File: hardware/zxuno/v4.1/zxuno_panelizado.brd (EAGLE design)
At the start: 103 parts, among them T1 BC846, U1 6SLX9TQG144, U2 FLASH-SPI-25XXSMD1, U4 AD724, U5 50MHz, U6 3.3V, U7 1.2V, Y1 3.58M, Y2 4.43M

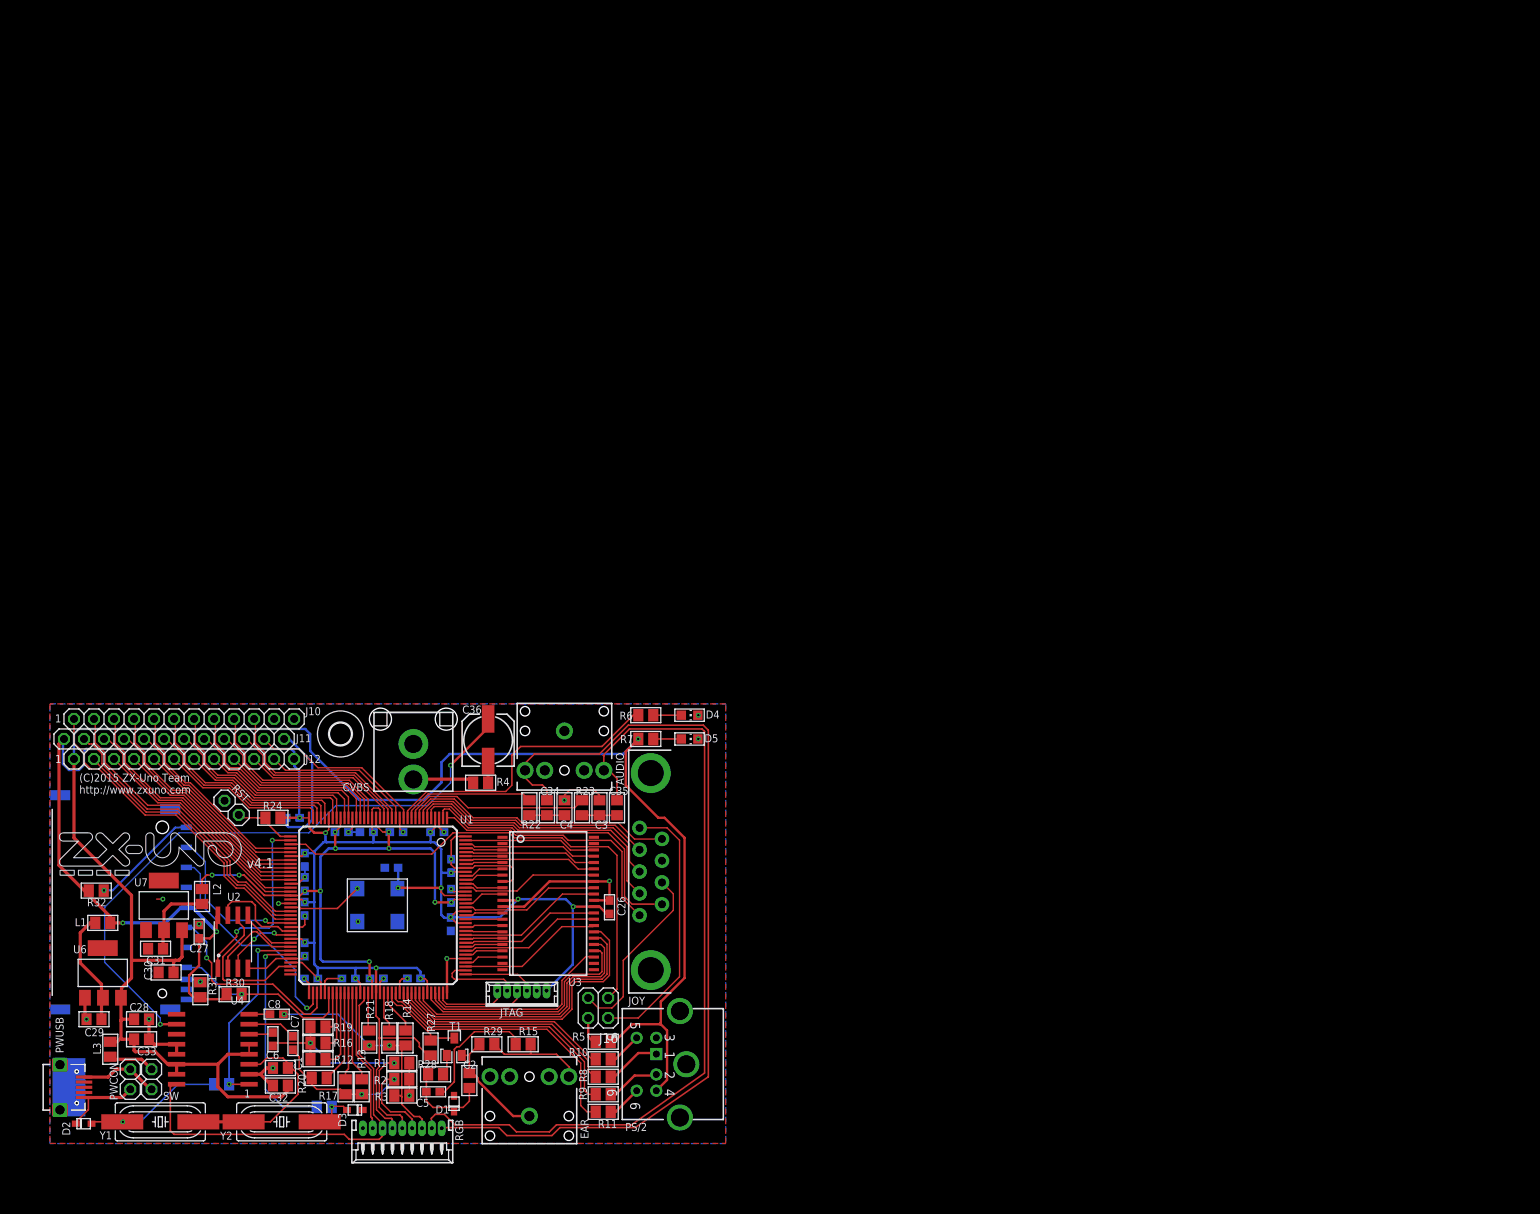
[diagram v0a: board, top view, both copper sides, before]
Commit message: Replico el circuito por 4 wire 0 (0 0) (190 0) (190 150) (0 150) (0 0) wire 0 (0 10) (190 10) wire 0 (0 140) (190 140)
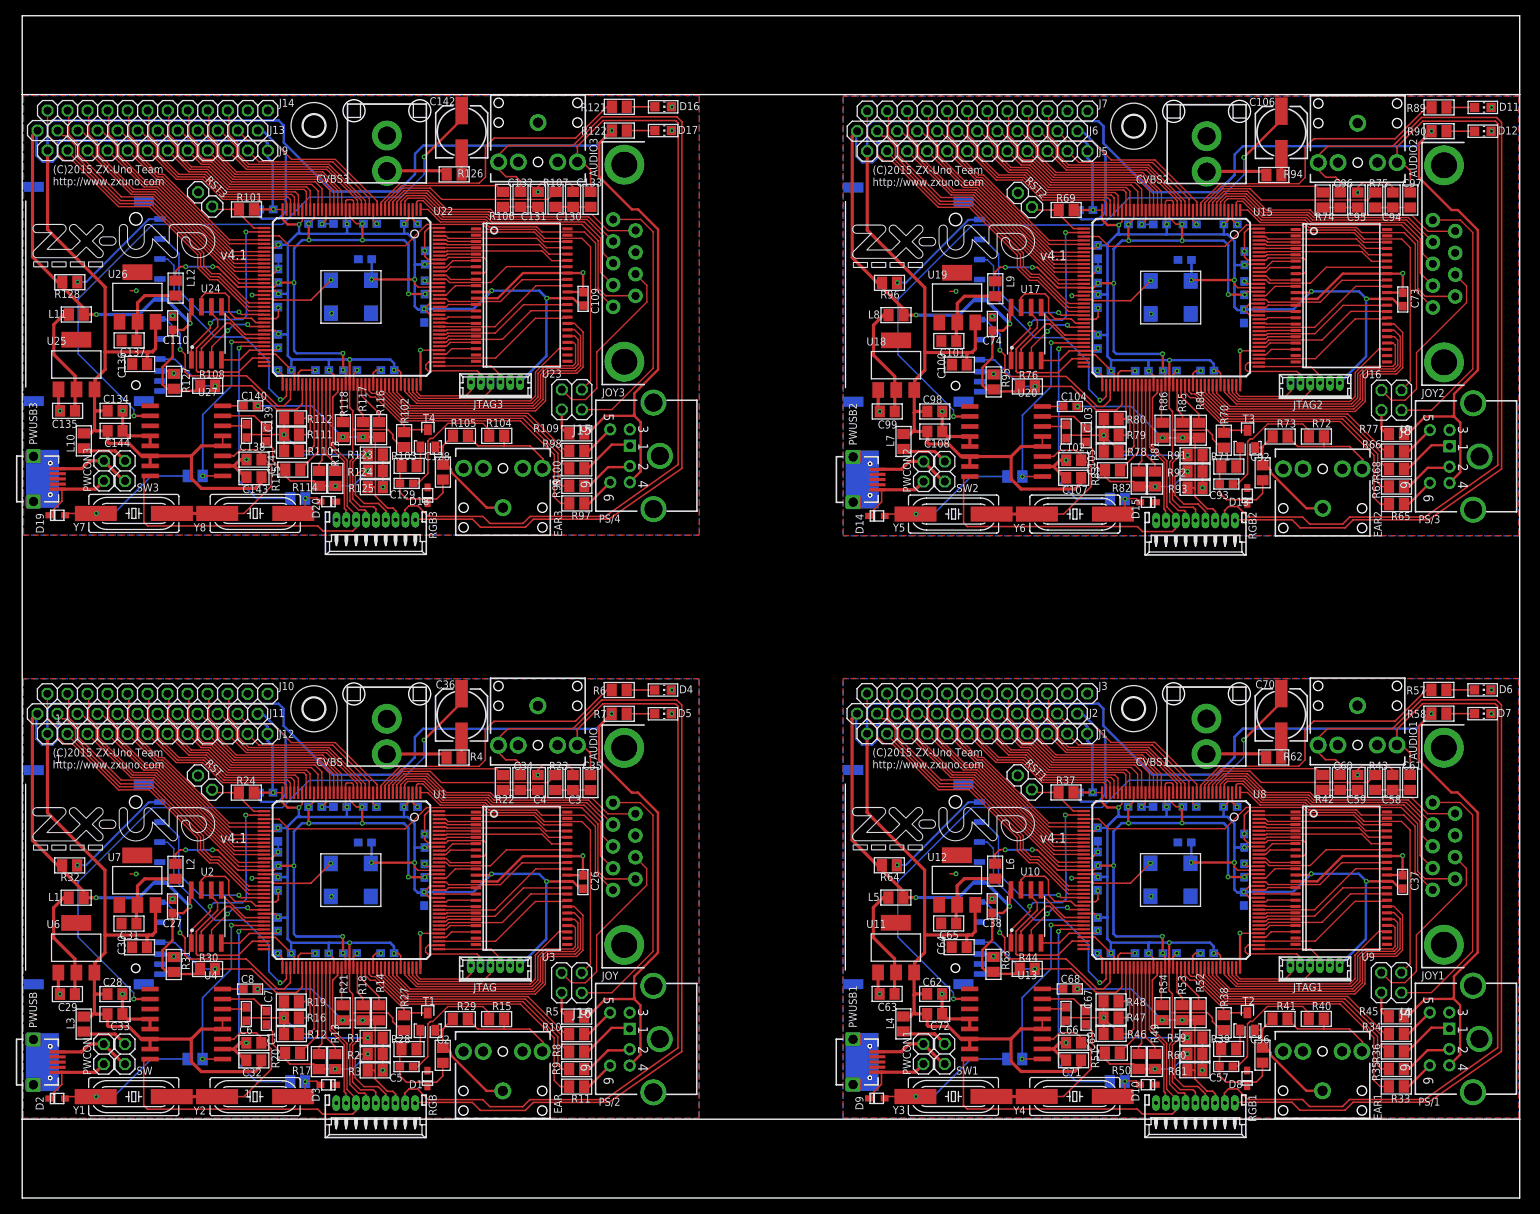
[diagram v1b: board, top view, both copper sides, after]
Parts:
- added AUDIO1, AUDIO2, AUDIO3: Audio, SparkFun-Connectors:AUDIO-JACK
- added C100, C101, C107, C108, C132, C133, C134, C135, C136, C137, C143, C144, C60, C61, C62, C63, C64, C65, C71, C72, C96, C97, C98, C99: 10uF, rcl:C0805
- added C102, C103, C104, C109, C110, C111, C112, C113, C114, C115, C116, C117, C118, C119, C120, C121, C122, C123, C124, C125, C126, C127, C129, C138, C139, C140, C37, C38, C39, C40, C41, C42, C43, C44, C45, C46, C47, C48, C49, C50, C51, C52, C53, C54, C55, C57, C66, C67, C68, C73, C74, C75, C76, C77, C78, C79, C80, C81, C82, C83, C84, C85, C86, C87, C88, C89, C90, C91, C93: 100nF, rcl:C0603
- added C105, C141, C69: 7.5pF, rcl:C0805
- added C106, C142, C70: 220uF, rcl:153CLV-0605
- added C128, C130, C131, C56, C58, C59, C92, C94, C95: 10nF, rcl:C0805
- added CVBS1, CVBS2, CVBS3: RCA, uzebox:RCA
- added D10, D13, D14, D15, D18, D19, D20, D8, D9: (no value), adafruit:SOD-323F
- added D11, D12, D16, D17, D6, D7: (no value), led:CHIP-LED0805
- added EAR1, EAR2, EAR3: EAR, SparkFun-Connectors:AUDIO-JACK
- added H2, H3, H4: MOUNT-HOLE2.8, holes:2,8
- added J1, J13, J14, J2, J3, J5, J6, J7, J9: (no value), pinhead:1X12
- added J15, J4, J8: (no value), pinhead:2X02
- added JOY1, JOY2, JOY3: (no value), SparkFun-Connectors:DB9_MALE
- added JTAG1, JTAG2, JTAG3: JTAG, con-molex:53047-06
- added L10, L11, L12, L4, L5, L6, L7, L8, L9: (no value), rcl:M0805
- added PS/1, PS/3, PS/4: PS/2 Keyb, ZX_UNO_0_14:DINC/MIN_TM/6_1PRIMARY
- added PWCON1, PWCON2, PWCON3, RST1, RST2, RST3, SW1, SW2, SW3: (no value), pinhead:1X02
- added PWUSB1, PWUSB2, PWUSB3: MICROUSB, zxuno_rev_mcleod:MICRO_USB_1PRIMARY
- added R100, R104, R109, R110, R113, R116, R121, R122, R33, R34, R35, R36, R40, R45, R46, R49, R52, R57, R58, R65, R66, R67, R68, R72, R77, R78, R81, R84, R89, R90, R97, R98, R99: 510, rcl:M0805
- added R101, R106, R107, R112, R115, R118, R37, R42, R43, R48, R51, R54, R69, R74, R75, R80, R83, R86: 2K, rcl:M0805
- added R102, R103, R105, R108, R119, R120, R127, R128, R38, R39, R41, R44, R55, R56, R63, R64, R70, R71, R73, R76, R87, R88, R95, R96: 10K, rcl:M0805
- added R111, R114, R117, R47, R50, R53, R79, R82, R85: 1K, rcl:M0805
- added R123, R124, R125, R126, R59, R60, R61, R62, R91, R92, R93, R94: 75, rcl:M0805
- added RGB1, RGB2, RGB3: RGB, con-molex:53048-09
- added SDCARD1, SDCARD2, SDCARD3: (no value), zxuno_rev_mcleod:SDCMF-10915W010
- added T2, T3, T4: BC846, transistor:SOT23
- added U10, U17, U24: FLASH-SPI-25XXSMD1, GadgetFactory:SO08-EIAJ
- added U11, U18, U25: 3.3V, burr-brown:SOT223
- added U12, U19, U26: 1.2V, burr-brown:SOT223
- added U13, U20, U27: AD724, ad725:SO16W
- added U14, U21, U28: 50MHz, ZX_UNO_0_15:SM/OSC_1PRIMARY
- added U15, U22, U8: 6SLX9TQG144, xilinx_devices_V6:TQ144
- added U16, U23, U9: (no value), GadgetFactory:TSOP44-II
- added Y3, Y5, Y7: 3.58M, crystal:HC49UP
- added Y4, Y6, Y8: 4.43M, crystal:HC49UP
- moved C26 4.65 mm to (71.1, 40.1)
- moved D4 4.65 mm to (81.3, 64.5)
- moved D5 4.65 mm to (81.3, 61.4)
- moved JOY 4.65 mm to (76.4, 44.6)
- moved R10 4.65 mm to (70.3, 20.8)
- moved R11 4.65 mm to (70.3, 14.1)
- moved R5 4.65 mm to (70.3, 23.0)
- moved R8 4.65 mm to (70.3, 18.6)
- moved R9 4.65 mm to (70.3, 16.4)
- moved AUDIO 4.65 mm to (65.4, 62.5)
- moved C11 4.65 mm to (51.0, 41.5)
- moved C13 4.65 mm to (32.5, 43.0)
- moved C23 4.65 mm to (32.5, 46.1)
- moved C34 4.65 mm to (63.2, 52.7)
- moved C35 4.65 mm to (72.1, 52.7)
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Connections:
- new net 1.2V1: C39.2, C40.2, C41.2, C42.2, C43.2, L6.2, U8.P128, U8.P19, U8.P28, U8.P52, U8.P89
- new net 1.2V2: C75.2, C76.2, C77.2, C78.2, C79.2, L9.2, U15.P128, U15.P19, U15.P28, U15.P52, U15.P89
- new net 1.2V3: C111.2, C112.2, C113.2, C114.2, C115.2, L12.2, U22.P128, U22.P19, U22.P28, U22.P52, U22.P89
- new net 3.3V1: C37.1, C38.2, C44.2, C45.2, C46.2, C47.2, C48.2, C49.2, C50.2, C51.2, C52.2, C53.2, C54.2, C55.2, J1.12, J2.1, JTAG1.1, L5.2, R37.2, R38.2, R44.1, R63.2, R64.2, RGB1.4, SDCARD1.4, U10.8, U14.4, U8.P103, U8.P122, U8.P125, U8.P129, U8.P135, U8.P18, U8.P20, U8.P31, U8.P36, U8.P4, U8.P42, U8.P53, U8.P63, U8.P69, U8.P76, U8.P86, U8.P90, U9.11, U9.33
- new net 3.3V2: C73.1, C74.2, C80.2, C81.2, C82.2, C83.2, C84.2, C85.2, C86.2, C87.2, C88.2, C89.2, C90.2, C91.2, J5.12, J6.1, JTAG2.1, L8.2, R69.2, R70.2, R76.1, R95.2, R96.2, RGB2.4, SDCARD2.4, U15.P103, U15.P122, U15.P125, U15.P129, U15.P135, U15.P18, U15.P20, U15.P31, U15.P36, U15.P4, U15.P42, U15.P53, U15.P63, U15.P69, U15.P76, U15.P86, U15.P90, U16.11, U16.33, U17.8, U21.4
- new net 3.3V3: C109.1, C110.2, C116.2, C117.2, C118.2, C119.2, C120.2, C121.2, C122.2, C123.2, C124.2, C125.2, C126.2, C127.2, J13.1, J9.12, JTAG3.1, L11.2, R101.2, R102.2, R108.1, R127.2, R128.2, RGB3.4, SDCARD3.4, U22.P103, U22.P122, U22.P125, U22.P129, U22.P135, U22.P18, U22.P20, U22.P31, U22.P36, U22.P4, U22.P42, U22.P53, U22.P63, U22.P69, U22.P76, U22.P86, U22.P90, U23.11, U23.33, U24.8, U28.4
- new net 5V1: C62.1, C64.1, C71.2, C72.2, J1.1, L4.2, PS/1.4, R45.1, R58.2, U11.3, U12.3, U13.14, U13.15, U13.4, U13.5
- new net 5V2: C100.1, C107.2, C108.2, C98.1, J5.1, L7.2, PS/3.4, R77.1, R90.2, U18.3, U19.3, U20.14, U20.15, U20.4, U20.5
- new net 5V3: C134.1, C136.1, C143.2, C144.2, J9.1, L10.2, PS/4.4, R109.1, R122.2, U25.3, U26.3, U27.14, U27.15, U27.4, U27.5
- new net AUDIO_LEFT1: R42.2, U8.P10
- new net AUDIO_LEFT2: R74.2, U15.P10
- new net AUDIO_LEFT3: R106.2, U22.P10
- new net AUDIO_RIGHT1: R43.2, U8.P9
- new net AUDIO_RIGHT2: R75.2, U15.P9
- new net AUDIO_RIGHT3: R107.2, U22.P9
- new net B10: C104.2, R84.1, R85.1, R86.1, R93.1, RGB2.7
- new net B11: R118.2, U22.P88
- new net B12: R117.2, U22.P92
- new net B13: R116.2, U22.P93
- new net B14: C140.2, R116.1, R117.1, R118.1, R125.1, RGB3.7
- new net B3: R54.2, U8.P88
- new net B4: R53.2, U8.P92
- new net B5: R52.2, U8.P93
- new net B6: C68.2, R52.1, R53.1, R54.1, R61.1, RGB1.7
- new net B7: R86.2, U15.P88
- new net B8: R85.2, U15.P92
- new net B9: R84.2, U15.P93
- new net CLK1: U14.3, U8.P55
- new net CLK2: U15.P55, U21.3
- new net CLK3: U22.P55, U28.3
- new net CSYNC1: RGB1.3, U13.16, U8.P87
- new net CSYNC2: RGB2.3, U15.P87, U20.16
- new net CSYNC3: RGB3.3, U22.P87, U27.16
- new net EAR1: R38.1, T2.3, U8.P94
- new net EAR2: R70.1, T3.3, U15.P94
- new net EAR3: R102.1, T4.3, U22.P94
- new net EXT1: J1.2, U8.P57
- new net EXT100: J9.5, U22.P43
- new net EXT101: J13.5, U22.P41
- new net EXT102: J14.5, U22.P40
- new net EXT103: J9.6, U22.P35
- new net EXT104: J13.6, U22.P34
- new net EXT105: J14.6, U22.P33
- new net EXT106: J9.7, U22.P32
- new net EXT107: J13.7, U22.P30
- new net EXT108: J14.7, U22.P29
- new net EXT109: J9.8, U22.P27
- new net EXT110: J13.8, U22.P26
- new net EXT111: J14.8, U22.P24
- new net EXT112: J9.9, U22.P23
- new net EXT113: J13.9, U22.P22
- new net EXT114: J14.9, U22.P21
- new net EXT115: J9.10, U22.P17
- new net EXT116: J13.10, U22.P16
- new net EXT117: J14.10, U22.P15
- new net EXT118: J9.11, U22.P14
- new net EXT119: J13.11, U22.P12
- new net EXT120: J14.1, U22.P58
- new net EXT2: J2.2, U8.P56
- new net EXT3: J3.2, U8.P51
- new net EXT36: J3.3, U8.P47
- new net EXT37: J1.4, U8.P46
- new net EXT38: J2.4, U8.P45
- new net EXT39: J3.4, U8.P44
- new net EXT4: J1.3, U8.P50
- new net EXT40: J1.5, U8.P43
- new net EXT41: J2.5, U8.P41
- new net EXT42: J3.5, U8.P40
- new net EXT43: J1.6, U8.P35
- new net EXT44: J2.6, U8.P34
- new net EXT45: J3.6, U8.P33
- new net EXT46: J1.7, U8.P32
- new net EXT47: J2.7, U8.P30
- new net EXT48: J3.7, U8.P29
- new net EXT49: J1.8, U8.P27
- new net EXT5: J2.3, U8.P48
- new net EXT50: J2.8, U8.P26
- new net EXT51: J3.8, U8.P24
- new net EXT52: J1.9, U8.P23
- new net EXT53: J2.9, U8.P22
- new net EXT54: J3.9, U8.P21
- new net EXT55: J1.10, U8.P17
- new net EXT56: J2.10, U8.P16
- new net EXT57: J3.10, U8.P15
- new net EXT58: J1.11, U8.P14
- new net EXT59: J2.11, U8.P12
- new net EXT60: J3.1, U8.P58
- new net EXT61: J5.2, U15.P57
- new net EXT62: J6.2, U15.P56
- new net EXT63: J7.2, U15.P51
- new net EXT64: J5.3, U15.P50
- new net EXT65: J6.3, U15.P48
- new net EXT66: J7.3, U15.P47
- new net EXT67: J5.4, U15.P46
- new net EXT68: J6.4, U15.P45
- new net EXT69: J7.4, U15.P44
- new net EXT70: J5.5, U15.P43
- new net EXT71: J6.5, U15.P41
- new net EXT72: J7.5, U15.P40
- new net EXT73: J5.6, U15.P35
- new net EXT74: J6.6, U15.P34
- new net EXT75: J7.6, U15.P33
- new net EXT76: J5.7, U15.P32
- new net EXT77: J6.7, U15.P30
- new net EXT78: J7.7, U15.P29
- new net EXT79: J5.8, U15.P27
- new net EXT80: J6.8, U15.P26
- new net EXT81: J7.8, U15.P24
- new net EXT82: J5.9, U15.P23
- new net EXT83: J6.9, U15.P22
- new net EXT84: J7.9, U15.P21
- new net EXT85: J5.10, U15.P17
- new net EXT86: J6.10, U15.P16
- new net EXT87: J7.10, U15.P15
- new net EXT88: J5.11, U15.P14
- new net EXT89: J6.11, U15.P12
- new net EXT90: J7.1, U15.P58
- new net EXT91: J9.2, U22.P57
- new net EXT92: J13.2, U22.P56
- new net EXT93: J14.2, U22.P51
- new net EXT94: J9.3, U22.P50
- new net EXT95: J13.3, U22.P48
- new net EXT96: J14.3, U22.P47
- new net EXT97: J9.4, U22.P46
- new net EXT98: J13.4, U22.P45
- new net EXT99: J14.4, U22.P44
- new net FLASH_CS1: U10.1, U8.P38
- new net FLASH_CS2: U15.P38, U17.1
- new net FLASH_CS3: U22.P38, U24.1
- new net FLASH_HOLD1: U10.7, U8.P61
- new net FLASH_HOLD2: U15.P61, U17.7
- new net FLASH_HOLD3: U22.P61, U24.7
- new net FLASH_MISO1: U10.2, U8.P65
- new net FLASH_MISO2: U15.P65, U17.2
- new net FLASH_MISO3: U22.P65, U24.2
- new net FLASH_MOSI1: U10.5, U8.P64
- new net FLASH_MOSI2: U15.P64, U17.5
- new net FLASH_MOSI3: U22.P64, U24.5
- new net FLASH_SCK1: U10.6, U8.P70
- new net FLASH_SCK2: U15.P70, U17.6
- new net FLASH_SCK3: U22.P70, U24.6
- new net FLASH_WP1: U10.3, U8.P62
- new net FLASH_WP2: U15.P62, U17.3
- new net FLASH_WP3: U22.P62, U24.3
- new net G10: C103.2, R81.1, R82.1, R83.1, R92.1, RGB2.6
- new net G11: R115.2, U22.P82
- new net G12: R114.2, U22.P83
- new net G13: R113.2, U22.P84
- new net G14: C139.2, R113.1, R114.1, R115.1, R124.1, RGB3.6
- new net G3: R51.2, U8.P82
- new net G4: R50.2, U8.P83
- new net G5: R49.2, U8.P84
- new net G6: C67.2, R49.1, R50.1, R51.1, R60.1, RGB1.6
- new net G7: R83.2, U15.P82
- new net G8: R82.2, U15.P83
- new net G9: R81.2, U15.P84
- new net GND1: AUDIO1.SLEEVE, C37.2, C38.1, C39.1, C40.1, C41.1, C42.1, C43.1, C44.1, C45.1, C46.1, C47.1, C48.1, C49.1, C50.1, C51.1, C52.1, C53.1, C54.1, C55.1, C56.2, C58.2, C59.2, C62.2, C63.2, C64.2, C65.2, C69.2, C71.1, C72.1, CVBS1.GND, D10.C, D6.C, D7.C, D8.A, D9.C, EAR1.SLEEVE, J2.12, J3.12, JOY1.8, JTAG1.2, PS/1.3, PWCON1.1, PWUSB1.5, R41.2, R59.2, R60.2, R61.2, RGB1.1, RST1.1, SDCARD1.3, SDCARD1.6, SDCARD1.M1, SDCARD1.M2, SDCARD1.M3, SDCARD1.M4, T2.2, U10.4, U11.1, U12.1, U13.12, U13.13, U13.2, U14.2, U8.P108, U8.P113, U8.P13, U8.P130, U8.P136, U8.P144, U8.P25, U8.P3, U8.P49, U8.P54, U8.P60, U8.P68, U8.P73, U8.P77, U8.P91, U8.P96, U9.12, U9.34, U9.37, U9.8
- new net GND2: AUDIO2.SLEEVE, C100.2, C101.2, C105.2, C107.1, C108.1, C73.2, C74.1, C75.1, C76.1, C77.1, C78.1, C79.1, C80.1, C81.1, C82.1, C83.1, C84.1, C85.1, C86.1, C87.1, C88.1, C89.1, C90.1, C91.1, C92.2, C94.2, C95.2, C98.2, C99.2, CVBS2.GND, D11.C, D12.C, D13.A, D14.C, D15.C, EAR2.SLEEVE, J6.12, J7.12, JOY2.8, JTAG2.2, PS/3.3, PWCON2.1, PWUSB2.5, R73.2, R91.2, R92.2, R93.2, RGB2.1, RST2.1, SDCARD2.3, SDCARD2.6, SDCARD2.M1, SDCARD2.M2, SDCARD2.M3, SDCARD2.M4, T3.2, U15.P108, U15.P113, U15.P13, U15.P130, U15.P136, U15.P144, U15.P25, U15.P3, U15.P49, U15.P54, U15.P60, U15.P68, U15.P73, U15.P77, U15.P91, U15.P96, U16.12, U16.34, U16.37, U16.8, U17.4, U18.1, U19.1, U20.12, U20.13, U20.2, U21.2
- new net GND3: AUDIO3.SLEEVE, C109.2, C110.1, C111.1, C112.1, C113.1, C114.1, C115.1, C116.1, C117.1, C118.1, C119.1, C120.1, C121.1, C122.1, C123.1, C124.1, C125.1, C126.1, C127.1, C128.2, C130.2, C131.2, C134.2, C135.2, C136.2, C137.2, C141.2, C143.1, C144.1, CVBS3.GND, D16.C, D17.C, D18.A, D19.C, D20.C, EAR3.SLEEVE, J13.12, J14.12, JOY3.8, JTAG3.2, PS/4.3, PWCON3.1, PWUSB3.5, R105.2, R123.2, R124.2, R125.2, RGB3.1, RST3.1, SDCARD3.3, SDCARD3.6, SDCARD3.M1, SDCARD3.M2, SDCARD3.M3, SDCARD3.M4, T4.2, U22.P108, U22.P113, U22.P13, U22.P130, U22.P136, U22.P144, U22.P25, U22.P3, U22.P49, U22.P54, U22.P60, U22.P68, U22.P73, U22.P77, U22.P91, U22.P96, U23.12, U23.34, U23.37, U23.8, U24.4, U25.1, U26.1, U27.12, U27.13, U27.2, U28.2
- new net JOY_DOWN1: JOY1.2, U8.P5
- new net JOY_DOWN2: JOY2.2, U15.P5
- new net JOY_DOWN3: JOY3.2, U22.P5
- new net JOY_FIRE10: JOY3.6, U22.P2
- new net JOY_FIRE11: JOY3.9, U22.P8
- new net JOY_FIRE12: J15.1, U22.P39
- new net JOY_FIRE4: JOY1.6, U8.P2
- new net JOY_FIRE5: JOY1.9, U8.P8
- new net JOY_FIRE6: J4.1, U8.P39
- new net JOY_FIRE7: JOY2.6, U15.P2
- new net JOY_FIRE8: JOY2.9, U15.P8
- new net JOY_FIRE9: J8.1, U15.P39
- new net JOY_LEFT1: JOY1.3, U8.P6
- new net JOY_LEFT2: JOY2.3, U15.P6
- new net JOY_LEFT3: JOY3.3, U22.P6
- new net JOY_RIGHT1: JOY1.4, U8.P7
- new net JOY_RIGHT2: JOY2.4, U15.P7
- new net JOY_RIGHT3: JOY3.4, U22.P7
- new net JOY_UP1: JOY1.1, U8.P1
- new net JOY_UP2: JOY2.1, U15.P1
- new net JOY_UP3: JOY3.1, U22.P1
- new net L-OUT1: AUDIO1.TIP, C60.2, RGB1.9
- new net L-OUT2: AUDIO2.TIP, C96.2, RGB2.9
- new net L-OUT3: AUDIO3.TIP, C132.2, RGB3.9
- new net LED1: R57.2, U8.P11
- new net LED2: R89.2, U15.P11
- new net LED3: R121.2, U22.P11
- new net N$100: C135.1, L11.1, U25.2
- new net N$101: C137.1, L12.1, U26.2
- new net N$102: C139.1, U27.7
- new net N$103: C138.1, U27.6
- new net N$104: C141.1, U27.3, Y7.2, Y8.2
- new net N$105: D20.A, R120.1, Y8.1
- new net N$106: D19.A, R119.2, Y7.1
- new net N$107: C142.+, U27.10
- new net N$108: C140.1, U27.8
- new net N$109: C142.-, R126.1
- new net N$110: CVBS3.SIG, R126.2
- new net N$111: D16.A, R121.1
- new net N$112: D17.A, R122.1
- new net N$113: R101.1, RST3.2, U22.P37
- new net N$114: R127.1, SDCARD3.8
- new net N$115: R128.1, SDCARD3.9
- new net N$116: J15.4, R109.2
- new net N$16: PS/1.6, R33.1
- new net N$29: PS/1.5, R34.1
- new net N$30: PS/1.2, R35.1
- new net N$33: PS/1.1, R36.1
- new net N$34: R39.2, T2.1
- new net N$35: C56.1, C57.1, D8.C, R39.1
- new net N$36: C57.2, R40.2
- new net N$37: EAR1.TIP, R40.1, R41.1
- new net N$38: C58.1, C61.1, R43.1
- new net N$39: C59.1, C60.1, R42.1
- new net N$40: PWCON1.2, PWUSB1.1, SW1.2
- new net N$41: L4.1, SW1.1
- new net N$42: C63.1, L5.1, U11.2
- new net N$43: C65.1, L6.1, U12.2
- new net N$44: C67.1, U13.7
- new net N$45: C66.1, U13.6
- new net N$46: C69.1, U13.3, Y3.2, Y4.2
- new net N$47: D10.A, R56.1, Y4.1
- new net N$48: D9.A, R55.2, Y3.1
- new net N$49: C70.+, U13.10
- new net N$50: C68.1, U13.8
- new net N$51: C70.-, R62.1
- new net N$52: CVBS1.SIG, R62.2
- new net N$53: D6.A, R57.1
- new net N$54: D7.A, R58.1
- new net N$55: R37.1, RST1.2, U8.P37
- new net N$56: R63.1, SDCARD1.8
- new net N$57: R64.1, SDCARD1.9
- new net N$58: J4.4, R45.2
- new net N$59: PS/3.6, R65.1
- new net N$60: PS/3.5, R66.1
- new net N$61: PS/3.2, R67.1
- new net N$62: PS/3.1, R68.1
- new net N$63: R71.2, T3.1
- new net N$64: C92.1, C93.1, D13.C, R71.1
- new net N$65: C93.2, R72.2
- new net N$66: EAR2.TIP, R72.1, R73.1
- new net N$67: C94.1, C97.1, R75.1
- new net N$68: C95.1, C96.1, R74.1
- new net N$69: PWCON2.2, PWUSB2.1, SW2.2
- new net N$70: L7.1, SW2.1
- new net N$71: C99.1, L8.1, U18.2
- new net N$72: C101.1, L9.1, U19.2
- new net N$73: C103.1, U20.7
- new net N$74: C102.1, U20.6
- new net N$75: C105.1, U20.3, Y5.2, Y6.2
- new net N$76: D15.A, R88.1, Y6.1
- new net N$77: D14.A, R87.2, Y5.1
- new net N$78: C106.+, U20.10
- new net N$79: C104.1, U20.8
- new net N$80: C106.-, R94.1
- new net N$81: CVBS2.SIG, R94.2
- new net N$82: D11.A, R89.1
- new net N$83: D12.A, R90.1
- new net N$84: R69.1, RST2.2, U15.P37
- new net N$85: R95.1, SDCARD2.8
- new net N$86: R96.1, SDCARD2.9
- new net N$87: J8.4, R77.2
- new net N$88: PS/4.6, R97.1
- new net N$89: PS/4.5, R98.1
- new net N$90: PS/4.2, R99.1
- new net N$91: PS/4.1, R100.1
- new net N$92: R103.2, T4.1
- new net N$93: C128.1, C129.1, D18.C, R103.1
- new net N$94: C129.2, R104.2
- new net N$95: EAR3.TIP, R104.1, R105.1
- new net N$96: C130.1, C133.1, R107.1
- new net N$97: C131.1, C132.1, R106.1
- new net N$98: PWCON3.2, PWUSB3.1, SW3.2
- new net N$99: L10.1, SW3.1
- new net PIN1: J4.3, JOY1.7
- new net PIN2: J4.2, JOY1.5
- new net PIN3: J8.3, JOY2.7
- new net PIN4: J8.2, JOY2.5
- new net PIN6: J15.3, JOY3.7
- new net PIN8: J15.2, JOY3.5
- new net PS2_CLK1: R34.2, U8.P99
- new net PS2_CLK2: R66.2, U15.P99
- new net PS2_CLK3: R98.2, U22.P99
- new net PS2_DATA1: R36.2, U8.P98
- new net PS2_DATA2: R68.2, U15.P98
- new net PS2_DATA3: R100.2, U22.P98
- new net PS2_PIN1: R33.2, U8.P95
- new net PS2_PIN3: R35.2, U8.P97
- new net PS2_PIN4: R65.2, U15.P95
- new net PS2_PIN5: R67.2, U15.P97
- new net PS2_PIN7: R97.2, U22.P95
- new net PS2_PIN8: R99.2, U22.P97
- new net R-OUT1: AUDIO1.RING, C61.2, RGB1.8
- new net R-OUT2: AUDIO2.RING, C97.2, RGB2.8
- new net R-OUT3: AUDIO3.RING, C133.2, RGB3.8
- new net R10: C102.2, R78.1, R79.1, R80.1, R91.1, RGB2.5
- new net R11: R112.2, U22.P79
- new net R12: R111.2, U22.P80
- new net R13: R110.2, U22.P81
- new net R14: C138.2, R110.1, R111.1, R112.1, R123.1, RGB3.5
- new net R3: R48.2, U8.P79
- new net R4: R47.2, U8.P80
- new net R5: R46.2, U8.P81
- new net R6: C66.2, R46.1, R47.1, R48.1, R59.1, RGB1.5
- new net R7: R80.2, U15.P79
- new net R8: R79.2, U15.P80
- new net R9: R78.2, U15.P81
- new net SD_CS1: SDCARD1.1, U8.P59
- new net SD_CS2: SDCARD2.1, U15.P59
- new net SD_CS3: SDCARD3.1, U22.P59
- new net SD_MISO1: R44.2, SDCARD1.7, U8.P78
- new net SD_MISO2: R76.2, SDCARD2.7, U15.P78
- new net SD_MISO3: R108.2, SDCARD3.7, U22.P78
- new net SD_MOSI1: SDCARD1.2, U8.P74
- new net SD_MOSI2: SDCARD2.2, U15.P74
- new net SD_MOSI3: SDCARD3.2, U22.P74
- new net SD_SCK1: SDCARD1.5, U8.P75
- new net SD_SCK2: SDCARD2.5, U15.P75
- new net SD_SCK3: SDCARD3.5, U22.P75
- new net STDN1: R55.1, U13.1, U8.P66
- new net STDN2: R87.1, U15.P66, U20.1
- new net STDN3: R119.1, U22.P66, U27.1
- new net STDNB1: R56.2, U8.P67
- new net STDNB2: R88.2, U15.P67
- new net STDNB3: R120.2, U22.P67
- new net TCK1: JTAG1.3, U8.P109
- new net TCK2: JTAG2.3, U15.P109
- new net TCK3: JTAG3.3, U22.P109
- new net TDI1: JTAG1.5, U8.P110
- new net TDI2: JTAG2.5, U15.P110
- new net TDI3: JTAG3.5, U22.P110
- new net TDO1: JTAG1.4, U8.P106
- new net TDO2: JTAG2.4, U15.P106
- new net TDO3: JTAG3.4, U22.P106
- new net TMS1: JTAG1.6, U8.P107
- new net TMS2: JTAG2.6, U15.P107
- new net TMS3: JTAG3.6, U22.P107
- new net VSYNC1: RGB1.2, U8.P85
- new net VSYNC2: RGB2.2, U15.P85
- new net VSYNC3: RGB3.2, U22.P85
- new net WR1: U8.P121, U9.15
- new net WR2: U15.P121, U16.15
- new net WR3: U22.P121, U23.15
- new net XA21: U8.P141, U9.3
- new net XA22: U8.P137, U9.5
- new net XA23: U8.P134, U9.6
- new net XA24: U8.P133, U9.7
- new net XA25: U8.P120, U9.16
- new net XA26: U8.P118, U9.17
- new net XA27: U8.P116, U9.18
- new net XA28: U8.P114, U9.19
- new net XA29: U8.P112, U9.20
- new net XA30: U8.P104, U9.26
- new net XA31: U8.P102, U9.27
- new net XA32: U8.P101, U9.28
- new net XA33: U8.P100, U9.29
- new net XA34: U8.P111, U9.30
- new net XA35: U8.P131, U9.38
- new net XA36: U8.P138, U9.39
- new net XA37: U8.P140, U9.40
- new net XA38: U8.P142, U9.41
- new net XA39: U8.P105, U9.25
- new net XA40: U8.P143, U9.42
- new net XA41: U8.P139, U9.4
- new net XA42: U15.P141, U16.3
- new net XA43: U15.P137, U16.5
- new net XA44: U15.P134, U16.6
- new net XA45: U15.P133, U16.7
- new net XA46: U15.P120, U16.16
- new net XA47: U15.P118, U16.17
- new net XA48: U15.P116, U16.18
- new net XA49: U15.P114, U16.19
- new net XA50: U15.P112, U16.20
- new net XA51: U15.P104, U16.26
- new net XA52: U15.P102, U16.27
- new net XA53: U15.P101, U16.28
- new net XA54: U15.P100, U16.29
- new net XA55: U15.P111, U16.30
- new net XA56: U15.P131, U16.38
- new net XA57: U15.P138, U16.39
- new net XA58: U15.P140, U16.40
- new net XA59: U15.P142, U16.41
- new net XA60: U15.P105, U16.25
- new net XA61: U15.P143, U16.42
- new net XA62: U15.P139, U16.4
- new net XA63: U22.P141, U23.3
- new net XA64: U22.P137, U23.5
- new net XA65: U22.P134, U23.6
- new net XA66: U22.P133, U23.7
- new net XA67: U22.P120, U23.16
- new net XA68: U22.P118, U23.17
- new net XA69: U22.P116, U23.18
- new net XA70: U22.P114, U23.19
- new net XA71: U22.P112, U23.20
- new net XA72: U22.P104, U23.26
- new net XA73: U22.P102, U23.27
- new net XA74: U22.P101, U23.28
- new net XA75: U22.P100, U23.29
- new net XA76: U22.P111, U23.30
- new net XA77: U22.P131, U23.38
- new net XA78: U22.P138, U23.39
- new net XA79: U22.P140, U23.40
- new net XA80: U22.P142, U23.41
- new net XA81: U22.P105, U23.25
- new net XA82: U22.P143, U23.42
- new net XA83: U22.P139, U23.4
- new net XD10: U8.P124, U9.13
- new net XD11: U8.P123, U9.14
- new net XD12: U8.P115, U9.31
- new net XD13: U8.P117, U9.32
- new net XD14: U8.P119, U9.35
- new net XD15: U8.P126, U9.36
- new net XD16: U15.P132, U16.9
- new net XD17: U15.P127, U16.10
- new net XD18: U15.P124, U16.13
- new net XD19: U15.P123, U16.14
- new net XD20: U15.P115, U16.31
- new net XD21: U15.P117, U16.32
- new net XD22: U15.P119, U16.35
- new net XD23: U15.P126, U16.36
- new net XD24: U22.P132, U23.9
- new net XD25: U22.P127, U23.10
- new net XD26: U22.P124, U23.13
- new net XD27: U22.P123, U23.14
- new net XD28: U22.P115, U23.31
- new net XD29: U22.P117, U23.32
- new net XD30: U22.P119, U23.35
- new net XD31: U22.P126, U23.36
- new net XD8: U8.P132, U9.9
- new net XD9: U8.P127, U9.10
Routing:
- net 3.3V2: track 0.00 -> 288.5 mm, vias 0 -> 19
- net 3.3V3: track 0.00 -> 288.5 mm, vias 0 -> 19
- net 3.3V1: track 0.00 -> 288.5 mm, vias 0 -> 19
- net 5V3: track 0.00 -> 233.3 mm, vias 0 -> 1
- net 5V1: track 0.00 -> 233.3 mm, vias 0 -> 1
- net 5V2: track 0.00 -> 233.3 mm, vias 0 -> 1
- net GND3: track 0.00 -> 149.1 mm, vias 0 -> 25
- net GND2: track 0.00 -> 149.1 mm, vias 0 -> 25
- net GND1: track 0.00 -> 149.1 mm, vias 0 -> 25
- net L-OUT2: track 0.00 -> 112.9 mm
- net L-OUT1: track 0.00 -> 112.9 mm
- net L-OUT3: track 0.00 -> 112.9 mm
- net R-OUT2: track 0.00 -> 104.1 mm
- net R-OUT3: track 0.00 -> 104.1 mm
- net R-OUT1: track 0.00 -> 104.1 mm
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- added copper zone on layer 1, net GND1
- added copper zone on layer 16, net GND1
- added copper zone on layer 1, net GND2
- added copper zone on layer 16, net GND2
- added copper zone on layer 1, net GND3
- added copper zone on layer 16, net GND3
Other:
- board outline added: 190 x 150 mm

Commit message: wire 0 (0 66) (190 66) wire 0 (0 84) (190 84) wire 0 (86 10) (86 140) wire 0 (104 10) (104 140)
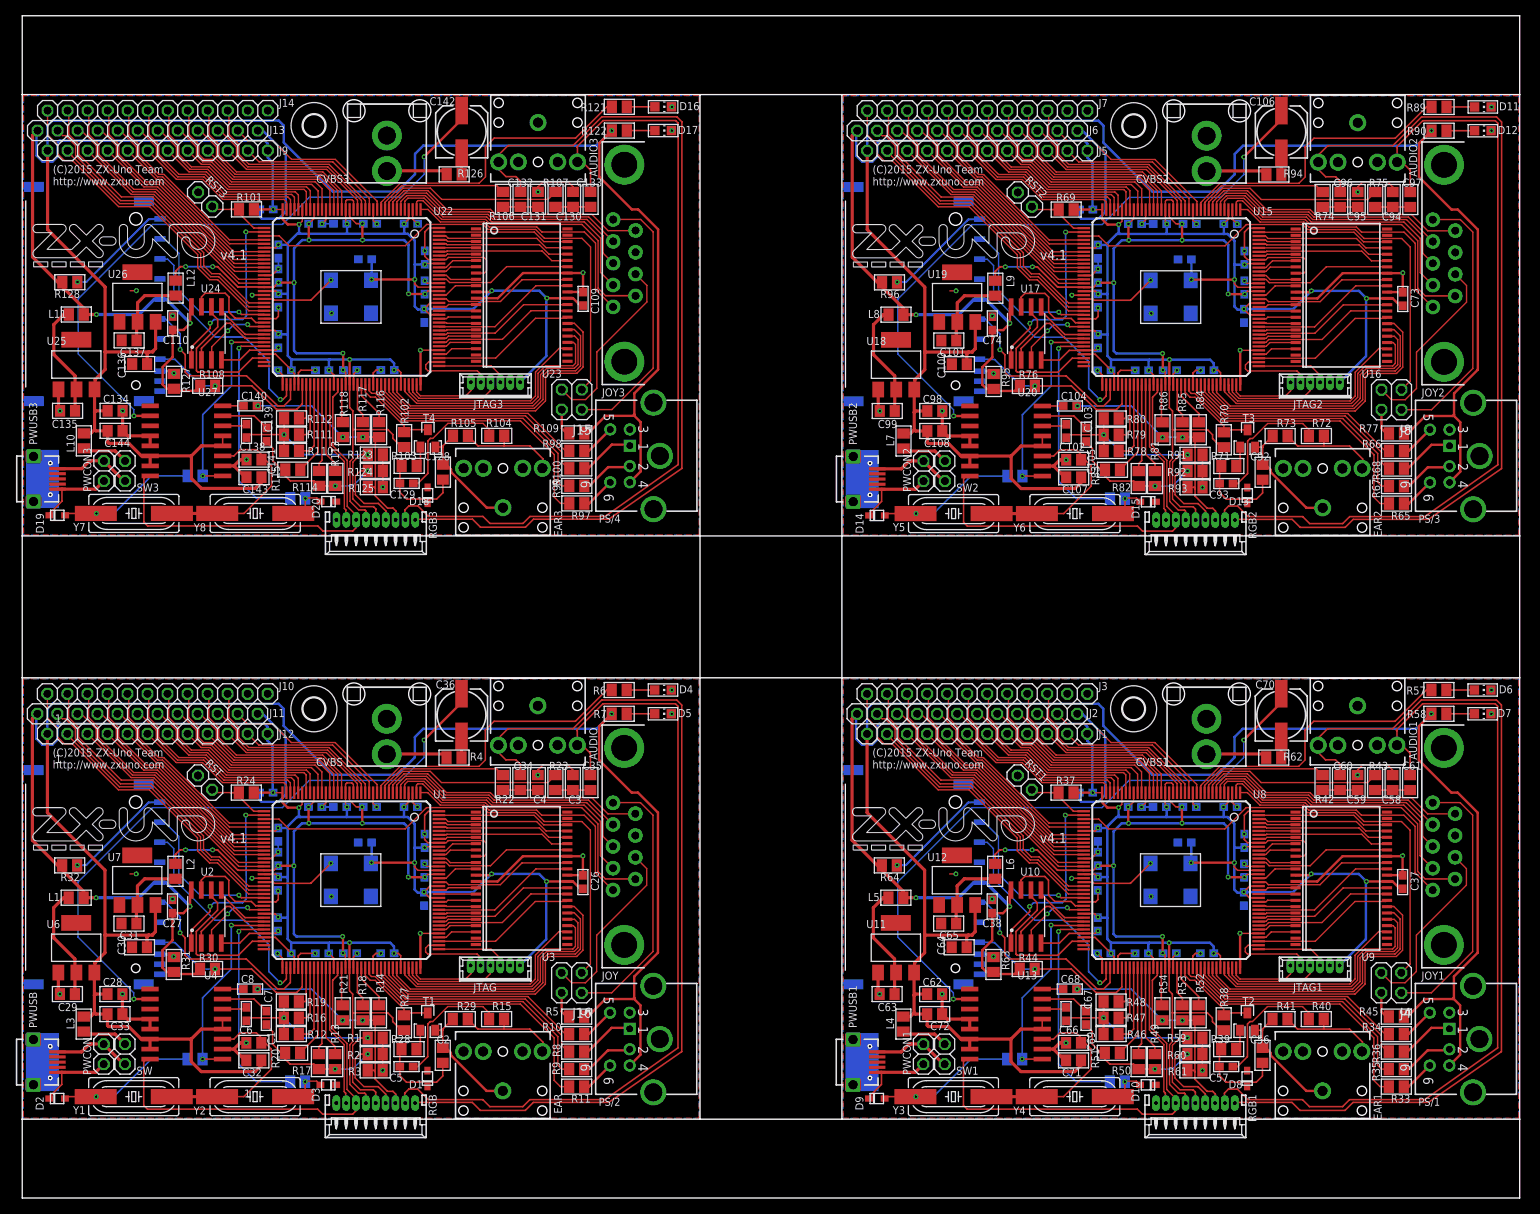
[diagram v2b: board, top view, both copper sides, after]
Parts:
- moved AUDIO2 0.06 mm to (169.4, 136.4)
- moved D11 0.06 mm to (185.3, 138.4)
- moved H3 0.06 mm to (141.0, 136.0)
- moved J7 0.06 mm to (121.2, 138.0)
- moved R89 0.06 mm to (179.8, 138.4)
- moved C101 0.06 mm to (117.6, 108.8)
- moved C103 0.06 mm to (135.0, 96.8)
- moved C73 0.06 mm to (175.2, 114.1)
- moved C74 0.06 mm to (123.1, 111.0)
- moved C75 0.06 mm to (141.2, 123.6)
- moved C76 0.06 mm to (148.1, 123.6)
- moved C77 0.06 mm to (155.1, 115.5)
- moved C79 0.06 mm to (136.5, 117.0)
- moved C80 0.06 mm to (144.3, 123.6)
- moved C81 0.06 mm to (153.3, 123.6)
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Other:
- outline, holes or cut-outs redrawn
